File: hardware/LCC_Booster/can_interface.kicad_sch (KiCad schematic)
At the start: 7 parts, among them U22 MCP2515-xSO, U23 MCP2562-E-SN, Y1 16.0 MHz, 22pF

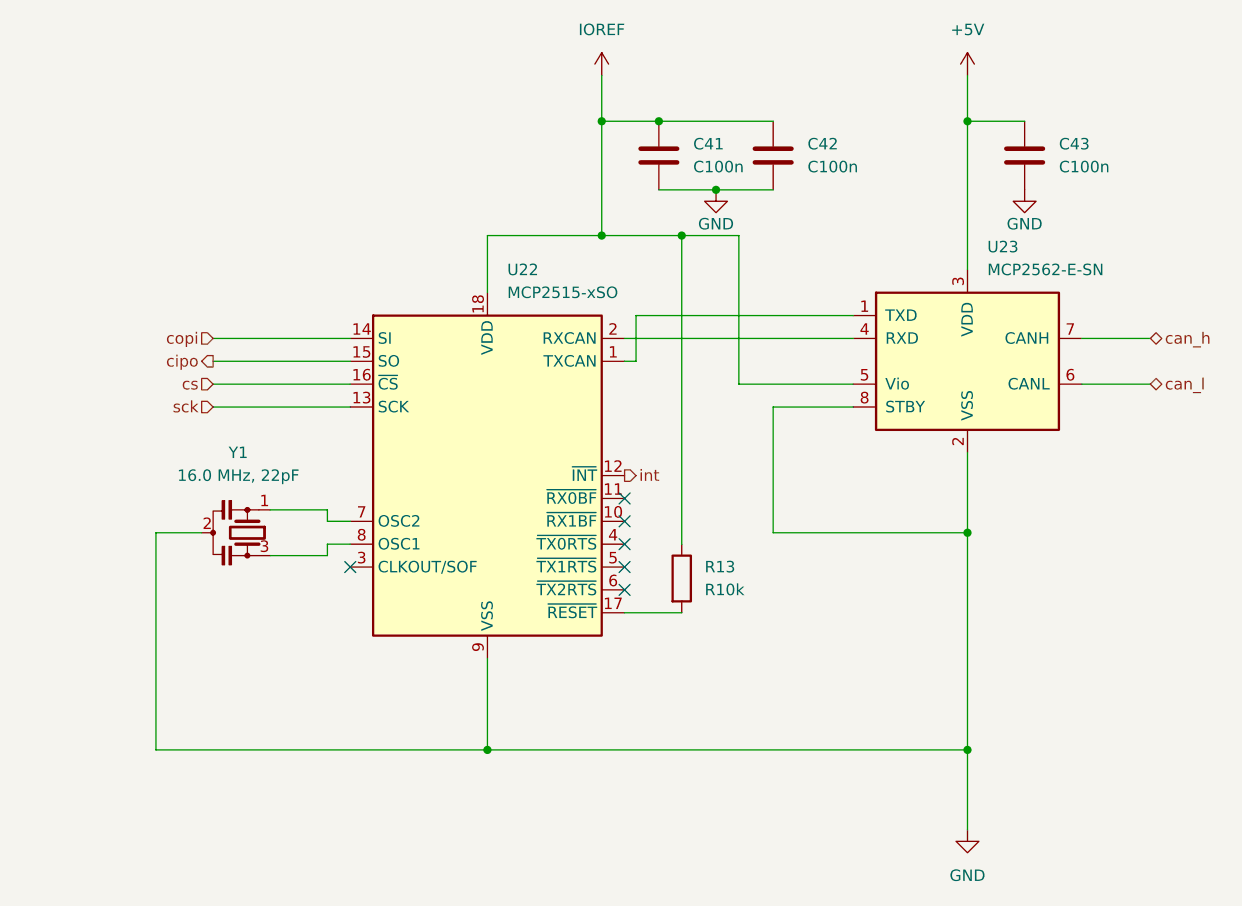
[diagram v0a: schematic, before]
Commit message: Better Solder Jumpers, Better Pizza
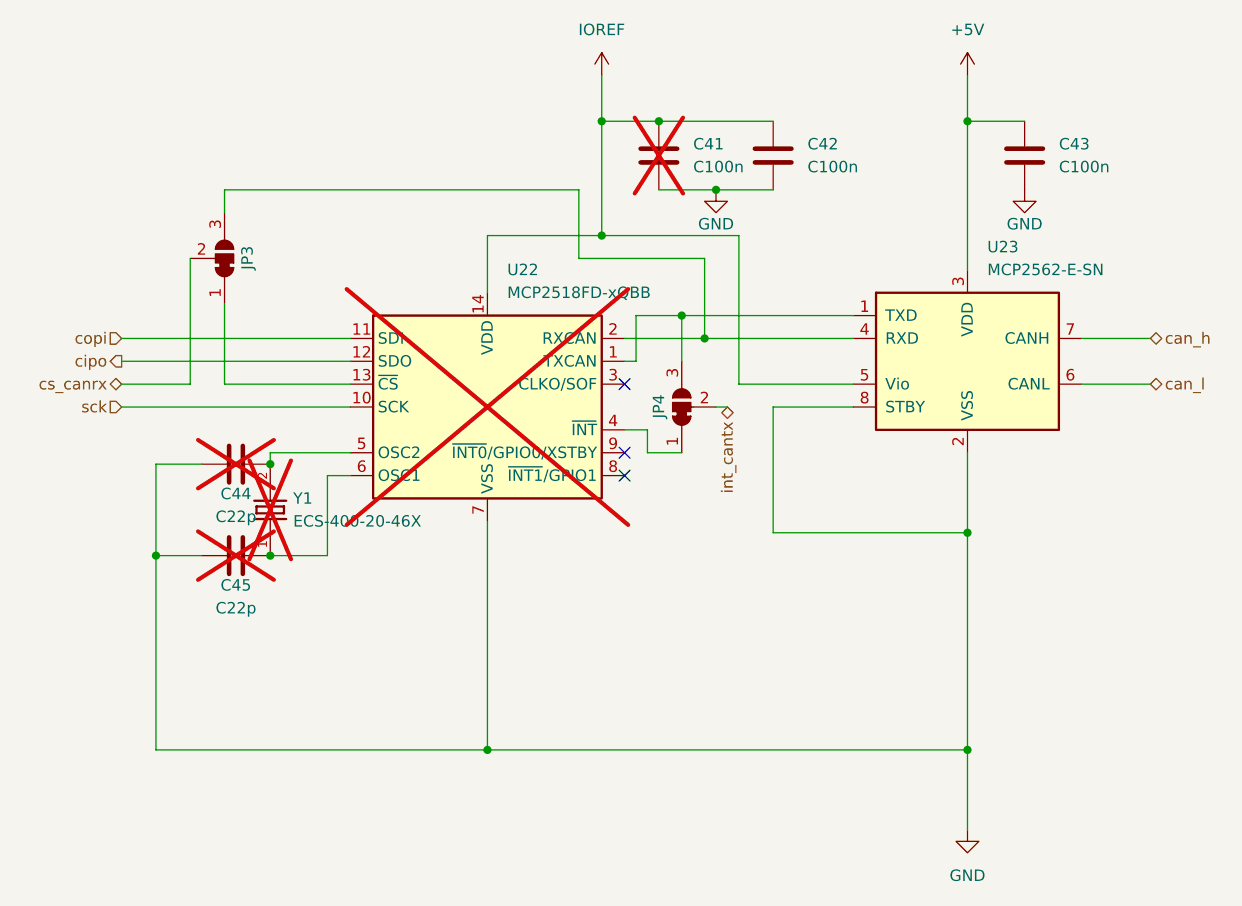
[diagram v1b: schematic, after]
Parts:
- removed R13: R10k, Resistor_SMD:R_01005_0402Metric_Pad0.57x0.30mm_HandSolder, symbol Device:R
- removed U22: MCP2515-xSO, Package_SO:SOIC-18W_7.5x11.6mm_P1.27mm, symbol Interface_CAN_LIN:MCP2515-xSO
- removed Y1: 16.0 MHz, 22pF, Crystal:Crystal_HC49-U-3Pin_Vertical, symbol Device:Resonator_Small
- added C44, C45: C22p, Capacitor_SMD:C_0402_1005Metric_Pad0.74x0.62mm_HandSolder, symbol Device:C
- added JP3, JP4: SolderJumper_3_Bridged12, Jumper:SolderJumper-3_P1.3mm_Bridged12_RoundedPad1.0x1.5mm_NumberLabels, symbol Jumper:SolderJumper_3_Bridged12
- added U22: MCP2518FD-xQBB, Package_SO:SOIC-14_3.9x8.7mm_P1.27mm, symbol Interface_CAN_LIN:MCP2518FD-xQBB
- added Y1: ECS-400-20-46X, ECS_400_20_46X:XTAL_ECS-400-20-46X, symbol ECS-400-20-46X:ECS-400-20-46X
- C41: now not fitted
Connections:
- net GND: now also C44.1, C45.1, U22.15 (VSS), U22.7 (VSS)
- net IOREF: now also U22.14 (VDD)
- net cipo: now also U22.12 (SDO)
- net copi: now also U22.11 (SDI)
- net sck: now also U22.10 (SCK)
- net at U23.1 (TXD): now also JP4.3 (B), U22.1 (TXCAN)
- net at U23.4 (RXD): now also JP3.3 (B), U22.2 (RXCAN)
- new net: C44.2, U22.5 (OSC2), Y1.2
- new net: JP4.1 (A), U22.4 (~{INT})
- new net: JP3.1 (A), U22.13 (~{CS})
- new net: C45.2, U22.6 (OSC1), Y1.1
- new net cs_canrx: JP3.2 (C)
- new net int_cantx: JP4.2 (C)
- no-connect marks 6 -> 3
